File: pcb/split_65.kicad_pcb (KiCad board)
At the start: 2 copper layers, 375 x 105.4 mm, 333 parts, among them J1 PJ-3200B-4A, J10 AVR-ISP-6, J11 Breakaway_Tabs, J12 Breakaway_Tabs, J13 Breakaway_Tabs, J14 Breakaway_Tabs, J15 Breakaway_Tabs, J16 Breakaway_Tabs, J2 AVR-ISP-6, J3 Breakaway_Tabs, J4 Breakaway_Tabs, J5 Breakaway_Tabs, J6 Breakaway_Tabs, J7 Breakaway_Tabs, J8 Breakaway_Tabs, J9 PJ-3200B-4A, Q1 2N7002, Q2 2N7002, SW1 SW_Push, SW2 SW_Push, U1 ATmega32U4-AU, U2 PRTR5V0U2X, U3 ATmega32U4-AU, U4 PRTR5V0U2X, Y1 16MHz, Y2 16MHz

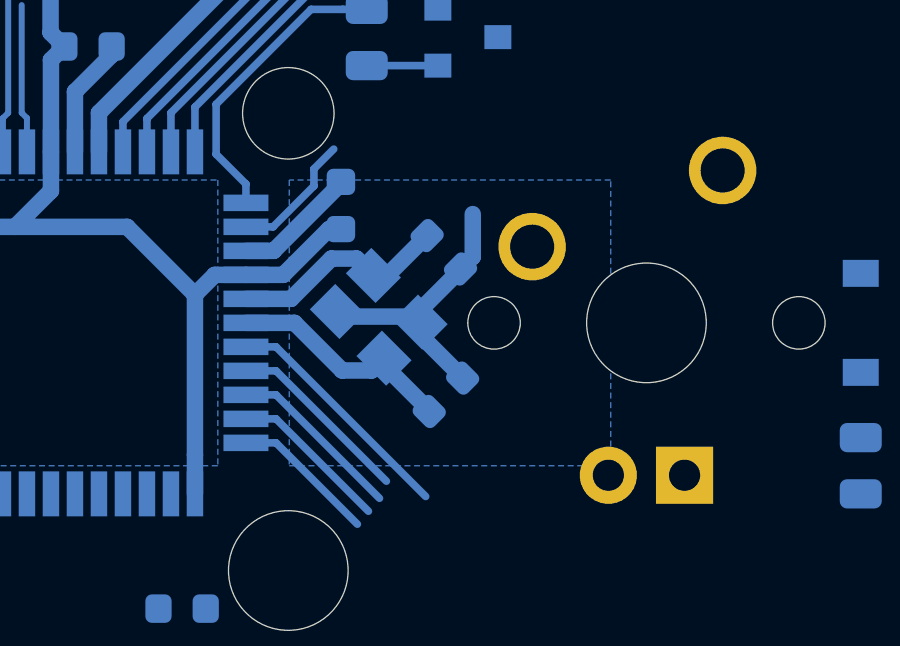
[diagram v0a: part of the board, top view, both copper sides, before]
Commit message: more traces
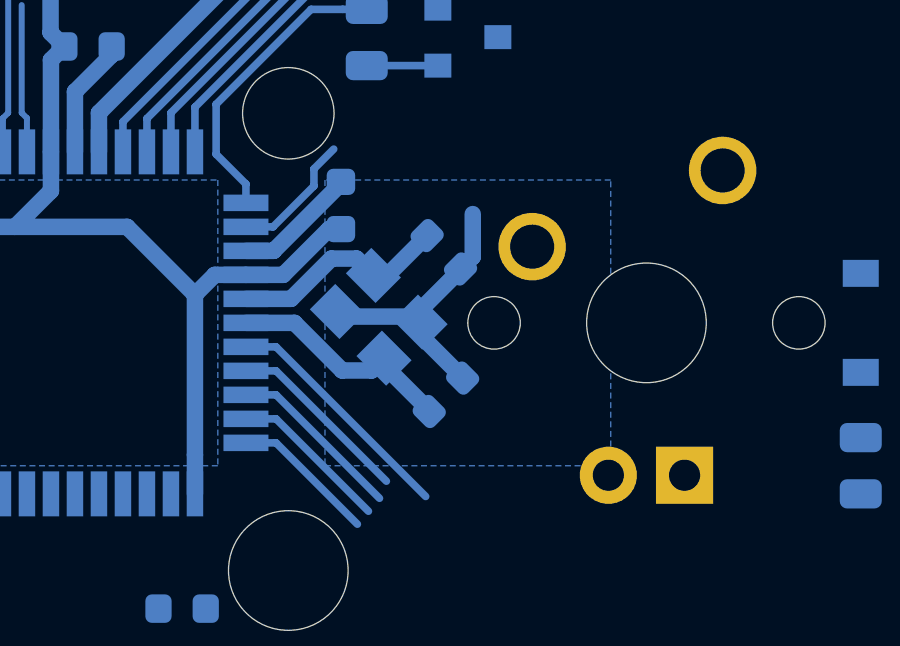
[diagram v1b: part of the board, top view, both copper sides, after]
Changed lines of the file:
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@@
   )
   (setup
-    (last_trace_width 0.55)
+    (last_trace_width 0.254)
     (user_trace_width 0.254)
     (user_trace_width 0.381)
@@
     (fp_line (start -0.8 0.4) (end 0.8 0.4) (layer B.Fab) (width 0.1))
     (fp_line (start -0.8 -0.4) (end -0.8 0.4) (layer B.Fab) (width 0.1))
-    (pad 2 smd roundrect (at 0.7875 0 45) (size 0.875 0.95) (layers B.Cu B.Paste B.Mask) (roundrect_rratio 0.25)
+    (pad 2 smd roundrect (at 0.787501 0 45) (size 0.875 0.95) (layers B.Cu B.Paste B.Mask) (roundrect_rratio 0.25)
       (net 1 GND))
-    (pad 1 smd roundrect (at -0.7875 0 45) (size 0.875 0.95) (layers B.Cu B.Paste B.Mask) (roundrect_rratio 0.25)
+    (pad 1 smd roundrect (at -0.787501 0 45) (size 0.875 0.95) (layers B.Cu B.Paste B.Mask) (roundrect_rratio 0.25)
       (net 2 "Net-(C1-Pad1)"))
     (model ${KISYS3DMOD}/Capacitor_SMD.3dshapes/C_0603_1608Metric.wrl
@@
     (polygon
       (pts
-        (xy 63.10339 123.82552) (xy 63.10339 114.30048) (xy 52.38772 114.30048) (xy 52.38772 123.82552)
+        (xy 63.10339 123.82552) (xy 63.10339 114.30048) (xy 53.57835 114.30048) (xy 53.57835 123.82552)
       )
     )
